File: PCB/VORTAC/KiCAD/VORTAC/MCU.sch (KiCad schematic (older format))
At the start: 43 parts, among them IC1 TMC2209-LA, U2 STM32F103C8Tx, U5 ADXL345BCCZ-RL7, U6 TJA1040T

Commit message: Added Protective Passives
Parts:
- removed D8: SK6812, LED_SMD:LED_SK6812_PLCC4_5.0x5.0mm_P3.2mm, symbol LED:SK6812
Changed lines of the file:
@@
 Text GLabel 700  4350 0    50   Input ~ 0
 TMC_DIAG
-Text GLabel 5100 5250 2    50   Input ~ 0
+Text GLabel 2050 4250 0    50   Input ~ 0
 FAN_1_TACHO
-Text GLabel 5100 5150 2    50   Input ~ 0
+Text GLabel 2050 4150 0    50   Input ~ 0
 FAN_2_TACHO
 Text GLabel 5100 5050 2    50   Input ~ 0
@@
 	1    0    0    -1
 $EndComp
-$Comp
-L LED:SK6812 D8
-U 1 1 61C17900
-P -300 3400
-F 0 "D8" H 44  3446 50  0000 L CNN
-F 1 "SK6812" H 44  3355 50  0000 L CNN
-F 2 "LED_SMD:LED_SK6812_PLCC4_5.0x5.0mm_P3.2mm" H -250 3100 50  0001 L TNN
-F 3 "https://cdn-shop.adafruit.com/product-files/1138/SK6812+LED+datasheet+.pdf" H -200 3025 50  0001 L TNN
-	1    -300 3400
-	1    0    0    -1
-$EndComp

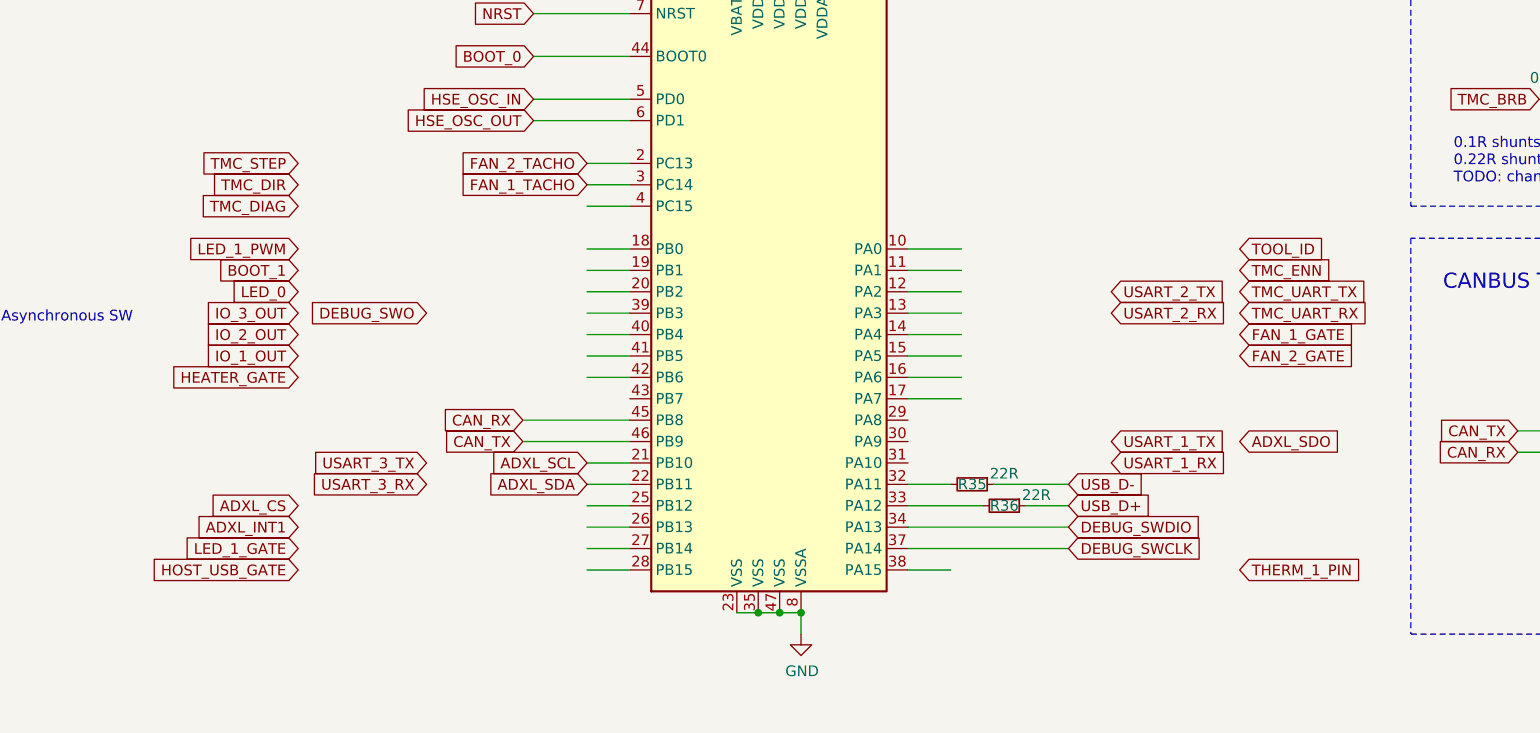
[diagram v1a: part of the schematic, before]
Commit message: Holiday Break <3
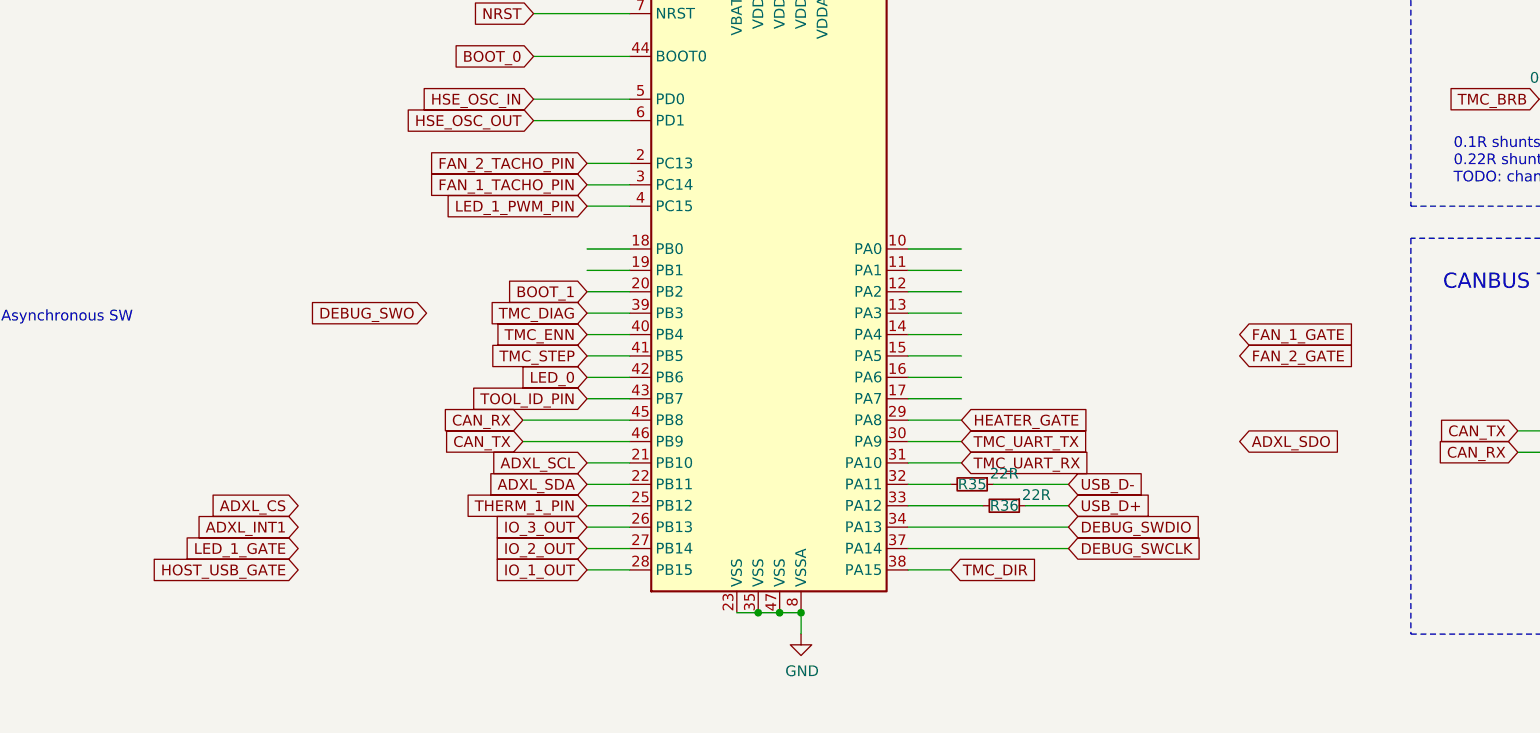
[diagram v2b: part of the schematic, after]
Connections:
- net labels added: FAN_1_TACHO_PIN, FAN_2_TACHO_PIN, LED_1_PWM_PIN, TOOL_ID_PIN
- net labels removed: FAN_1_TACHO, FAN_2_TACHO, LED_1_PWM, TOOL_ID, USART_1_RX, USART_1_TX, USART_2_RX, USART_2_TX, USART_3_RX, USART_3_TX
- wire segments 203 -> 207
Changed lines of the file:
@@
 Wire Wire Line
 	4100 5750 4300 5750
-Text GLabel 4500 5450 2    50   Input ~ 0
-USART_1_TX
-Text GLabel 4500 5550 2    50   Input ~ 0
-USART_1_RX
 Wire Wire Line
 	3550 5650 3750 5650
@@
 Wire Wire Line
 	3550 5750 3900 5750
-Text GLabel 1300 5550 0    50   Input ~ 0
-USART_3_TX
-Text GLabel 1300 5650 0    50   Input ~ 0
-USART_3_RX
 Wire Wire Line
 	2050 5550 2250 5550
@@
 Wire Wire Line
 	2050 4650 2250 4650
-Text GLabel 700  4250 0    50   Input ~ 0
+Text GLabel 3750 6050 2    50   Input ~ 0
 TMC_DIR
-Text GLabel 700  4150 0    50   Input ~ 0
+Text GLabel 2050 5050 0    50   Input ~ 0
 TMC_STEP
-Text GLabel 5100 4650 2    50   Input ~ 0
+Text GLabel 2050 4950 0    50   Input ~ 0
 TMC_ENN
-Text GLabel 700  4350 0    50   Input ~ 0
+Text GLabel 2050 4850 0    50   Input ~ 0
 TMC_DIAG
 Text GLabel 2050 4250 0    50   Input ~ 0
-FAN_1_TACHO
+FAN_1_TACHO_PIN
 Text GLabel 2050 4150 0    50   Input ~ 0
-FAN_2_TACHO
+FAN_2_TACHO_PIN
 Text GLabel 5100 5050 2    50   Input ~ 0
 FAN_2_GATE
-Text GLabel 700  5150 0    50   Input ~ 0
+Text GLabel 3800 5350 2    50   Input ~ 0
 HEATER_GATE
 Text GLabel 700  5950 0    50   Input ~ 0
@@
 Text GLabel 700  6050 0    50   Input ~ 0
 HOST_USB_GATE
-Text GLabel 700  4750 0    50   Input ~ 0
+Text GLabel 2050 5150 0    50   Input ~ 0
 LED_0
 Text GLabel 700  5750 0    50   Input ~ 0
@@
 Text GLabel 700  5850 0    50   Input ~ 0
 ADXL_INT1
-Text GLabel 5100 4550 2    50   Input ~ 0
-TOOL_ID
-Text GLabel 5100 6050 2    50   Input ~ 0
+Text GLabel 2050 5250 0    50   Input ~ 0
+TOOL_ID_PIN
+Text GLabel 2050 5750 0    50   Input ~ 0
 THERM_1_PIN
-Text GLabel 700  4850 0    50   Input ~ 0
+Text GLabel 2050 5850 0    50   Input ~ 0
 IO_3_OUT
-Text GLabel 700  4950 0    50   Input ~ 0
+Text GLabel 2050 5950 0    50   Input ~ 0
 IO_2_OUT
-Text GLabel 700  5050 0    50   Input ~ 0
+Text GLabel 2050 6050 0    50   Input ~ 0
 IO_1_OUT
 $Comp
@@
 	1    0    0    -1
 $EndComp
-Text GLabel 700  4650 0    50   Input ~ 0
+Text GLabel 2050 4750 0    50   Input ~ 0
 BOOT_1
 Wire Wire Line
@@
 Text GLabel 5100 4950 2    50   Input ~ 0
 FAN_1_GATE
-Text GLabel 4500 4850 2    50   Input ~ 0
-USART_2_RX
-Text GLabel 4500 4750 2    50   Input ~ 0
-USART_2_TX
-Text GLabel 700  4550 0    50   Input ~ 0
-LED_1_PWM
+Text GLabel 2050 4350 0    50   Input ~ 0
+LED_1_PWM_PIN
 Wire Wire Line
 	3550 4950 3800 4950
@@
 Wire Wire Line
 	2050 5150 2250 5150
-Text GLabel 5100 4850 2    50   Input ~ 0
+Text GLabel 3800 5550 2    50   Input ~ 0
 TMC_UART_RX
-Text GLabel 5100 4750 2    50   Input ~ 0
+Text GLabel 3800 5450 2    50   Input ~ 0
 TMC_UART_TX
 Wire Wire Line
@@
 $EndComp
 Connection ~ 1850 1350
+Wire Wire Line
+	2050 5250 2250 5250
+Wire Wire Line
+	3800 5350 3550 5350
+Wire Wire Line
+	3550 5450 3800 5450
+Wire Wire Line
+	3800 5550 3550 5550
 $EndSCHEMATC
